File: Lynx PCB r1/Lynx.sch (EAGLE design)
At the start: 105 parts, among them IC3 ICL7660, Q1 8MHz, X1 BU-SMA-V, X2 BU-SMA-V

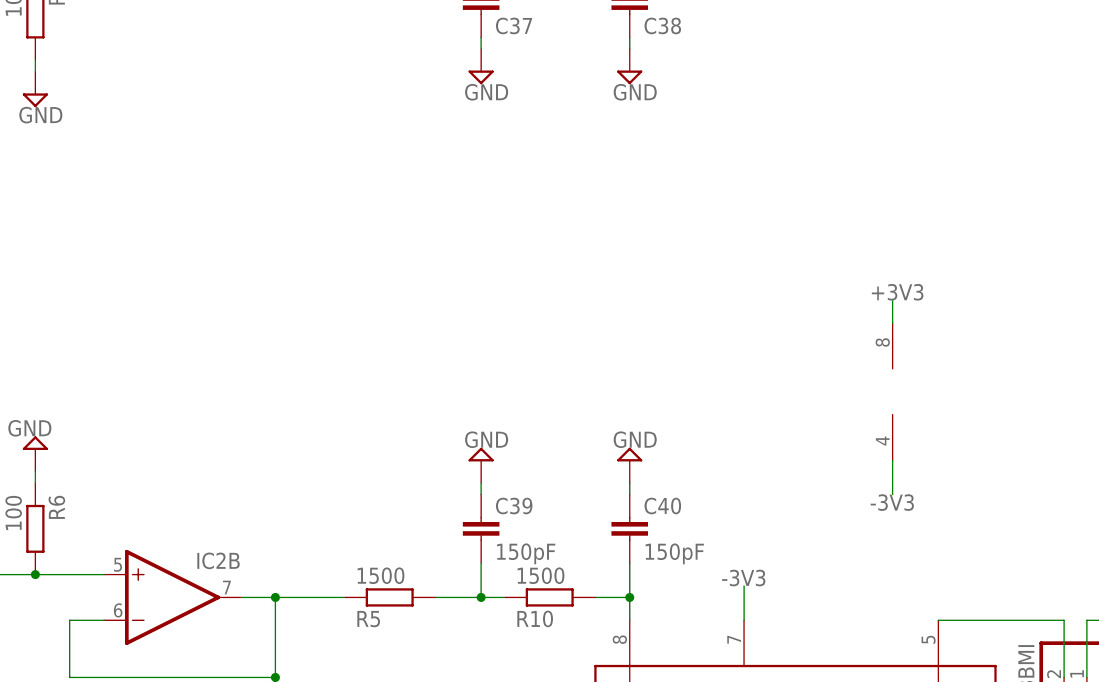
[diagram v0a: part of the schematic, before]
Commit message: All routed
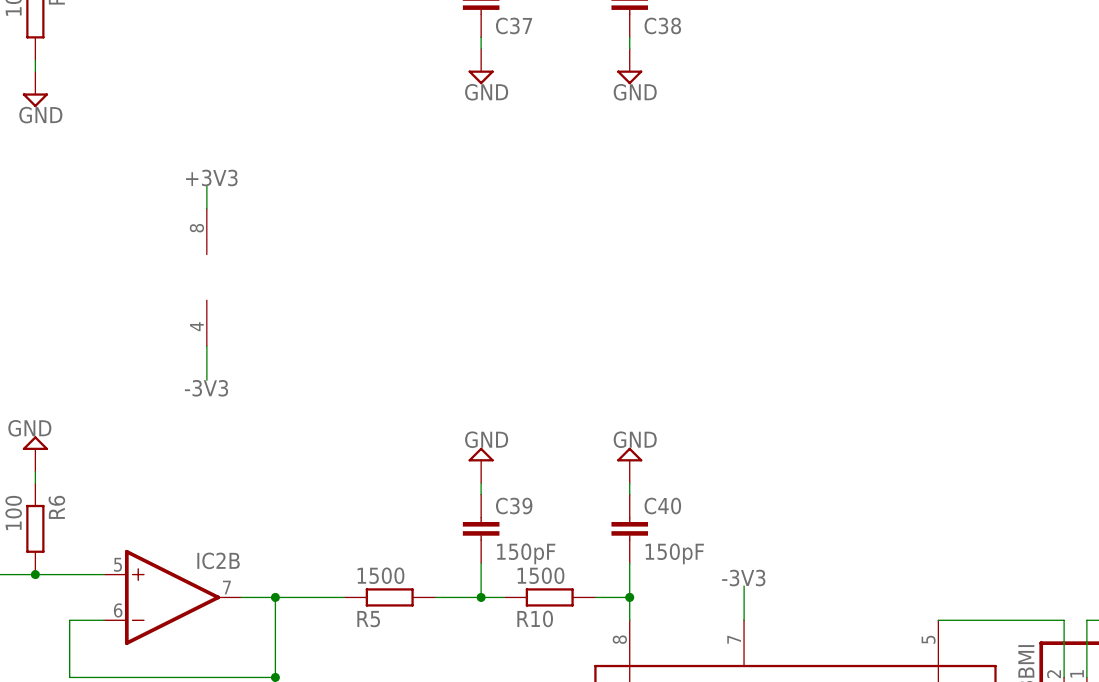
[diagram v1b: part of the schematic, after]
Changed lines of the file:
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@@
 <setting verticaltext="up"/>
 </settings>
-<grid distance="0.05" unitdist="inch" unit="inch" style="lines" multiple="1" display="no" altdistance="0.01" altunitdist="inch" altunit="inch"/>
+<grid distance="0.1" unitdist="inch" unit="inch" style="lines" multiple="1" display="no" altdistance="0.01" altunitdist="inch" altunit="inch"/>
 <layers>
-<layer number="1" name="Top" color="4" fill="1" visible="yes" active="no"/>
-<layer number="2" name="Route2" color="1" fill="3" visible="yes" active="no"/>
-<layer number="3" name="Route3" color="4" fill="3" visible="yes" active="no"/>
-<layer number="4" name="Route4" color="1" fill="4" visible="yes" active="no"/>
-<layer number="5" name="Route5" color="4" fill="4" visible="yes" active="no"/>
-<layer number="6" name="Route6" color="1" fill="8" visible="yes" active="no"/>
-<layer number="7" name="Route7" color="4" fill="8" visible="yes" active="no"/>
-<layer number="8" name="Route8" color="1" fill="2" visible="yes" active="no"/>
-<layer number="9" name="Route9" color="4" fill="2" visible="yes" active="no"/>
-<layer number="10" name="Route10" color="1" fill="7" visible="yes" active="no"/>
-<layer number="11" name="Route11" color="4" fill="7" visible="yes" active="no"/>
-<layer number="12" name="Route12" color="1" fill="5" visible="yes" active="no"/>
-<layer number="13" name="Route13" color="4" fill="5" visible="yes" active="no"/>
-<layer number="14" name="Route14" color="1" fill="6" visible="yes" active="no"/>
-<layer number="15" name="Route15" color="4" fill="6" visible="yes" active="no"/>
-<layer number="16" name="Bottom" color="1" fill="1" visible="yes" active="no"/>
-<layer number="17" name="Pads" color="2" fill="1" visible="yes" active="no"/>
-<layer number="18" name="Vias" color="2" fill="1" visible="yes" active="no"/>
-<layer number="19" name="Unrouted" color="6" fill="1" visible="yes" active="no"/>
-<layer number="20" name="Dimension" color="15" fill="1" visible="yes" active="no"/>
-<layer number="21" name="tPlace" color="7" fill="1" visible="yes" active="no"/>
-<layer number="22" name="bPlace" color="7" fill="1" visible="yes" active="no"/>
-<layer number="23" name="tOrigins" color="15" fill="1" visible="yes" active="no"/>
-<layer number="24" name="bOrigins" color="15" fill="1" visible="yes" active="no"/>
-<layer number="25" name="tNames" color="7" fill="1" visible="yes" active="no"/>
-<layer number="26" name="bNames" color="7" fill="1" visible="yes" active="no"/>
-<layer number="27" name="tValues" color="7" fill="1" visible="yes" active="no"/>
-<layer number="28" name="bValues" color="7" fill="1" visible="yes" active="no"/>
+<layer number="1" name="Top" color="4" fill="1" visible="no" active="no"/>
+<layer number="2" name="Route2" color="1" fill="3" visible="no" active="no"/>
+<layer number="3" name="Route3" color="4" fill="3" visible="no" active="no"/>
+<layer number="4" name="Route4" color="1" fill="4" visible="no" active="no"/>
+<layer number="5" name="Route5" color="4" fill="4" visible="no" active="no"/>
+<layer number="6" name="Route6" color="1" fill="8" visible="no" active="no"/>
+<layer number="7" name="Route7" color="4" fill="8" visible="no" active="no"/>
+<layer number="8" name="Route8" color="1" fill="2" visible="no" active="no"/>
+<layer number="9" name="Route9" color="4" fill="2" visible="no" active="no"/>
+<layer number="10" name="Route10" color="1" fill="7" visible="no" active="no"/>
+<layer number="11" name="Route11" color="4" fill="7" visible="no" active="no"/>
+<layer number="12" name="Route12" color="1" fill="5" visible="no" active="no"/>
+<layer number="13" name="Route13" color="4" fill="5" visible="no" active="no"/>
+<layer number="14" name="Route14" color="1" fill="6" visible="no" active="no"/>
+<layer number="15" name="Route15" color="4" fill="6" visible="no" active="no"/>
+<layer number="16" name="Bottom" color="1" fill="1" visible="no" active="no"/>
+<layer number="17" name="Pads" color="2" fill="1" visible="no" active="no"/>
+<layer number="18" name="Vias" color="2" fill="1" visible="no" active="no"/>
+<layer number="19" name="Unrouted" color="6" fill="1" visible="no" active="no"/>
+<layer number="20" name="Dimension" color="15" fill="1" visible="no" active="no"/>
+<layer number="21" name="tPlace" color="7" fill="1" visible="no" active="no"/>
+<layer number="22" name="bPlace" color="7" fill="1" visible="no" active="no"/>
+<layer number="23" name="tOrigins" color="15" fill="1" visible="no" active="no"/>
+<layer number="24" name="bOrigins" color="15" fill="1" visible="no" active="no"/>
+<layer number="25" name="tNames" color="7" fill="1" visible="no" active="no"/>
+<layer number="26" name="bNames" color="7" fill="1" visible="no" active="no"/>
+<layer number="27" name="tValues" color="7" fill="1" visible="no" active="no"/>
+<layer number="28" name="bValues" color="7" fill="1" visible="no" active="no"/>
 <layer number="29" name="tStop" color="7" fill="3" visible="no" active="no"/>
 <layer number="30" name="bStop" color="7" fill="6" visible="no" active="no"/>
@@
 <layer number="35" name="tGlue" color="7" fill="4" visible="no" active="no"/>
 <layer number="36" name="bGlue" color="7" fill="5" visible="no" active="no"/>
-<layer number="37" name="tTest" color="7" fill="1" visible="yes" active="no"/>
-<layer number="38" name="bTest" color="7" fill="1" visible="yes" active="no"/>
+<layer number="37" name="tTest" color="7" fill="1" visible="no" active="no"/>
+<layer number="38" name="bTest" color="7" fill="1" visible="no" active="no"/>
 <layer number="39" name="tKeepout" color="4" fill="11" visible="no" active="no"/>
 <layer number="40" name="bKeepout" color="1" fill="11" visible="no" active="no"/>
@@
 <layer number="44" name="Drills" color="7" fill="1" visible="no" active="no"/>
 <layer number="45" name="Holes" color="7" fill="1" visible="no" active="no"/>
-<layer number="46" name="Milling" color="3" fill="1" visible="yes" active="no"/>
-<layer number="47" name="Measures" color="7" fill="1" visible="yes" active="no"/>
-<layer number="48" name="Document" color="7" fill="1" visible="yes" active="no"/>
-<layer number="49" name="Reference" color="7" fill="1" visible="yes" active="no"/>
-<layer number="50" name="dxf" color="7" fill="1" visible="yes" active="no"/>
-<layer number="51" name="tDocu" color="7" fill="1" visible="yes" active="no"/>
-<layer number="52" name="bDocu" color="7" fill="1" visible="yes" active="no"/>
-<layer number="53" name="tGND_GNDA" color="7" fill="9" visible="yes" active="no"/>
-<layer number="54" name="bGND_GNDA" color="1" fill="9" visible="yes" active="no"/>
-<layer number="56" name="wert" color="7" fill="1" visible="yes" active="no"/>
+<layer number="46" name="Milling" color="3" fill="1" visible="no" active="no"/>
+<layer number="47" name="Measures" color="7" fill="1" visible="no" active="no"/>
+<layer number="48" name="Document" color="7" fill="1" visible="no" active="no"/>
+<layer number="49" name="Reference" color="7" fill="1" visible="no" active="no"/>
+<layer number="50" name="dxf" color="7" fill="1" visible="no" active="no"/>
+<layer number="51" name="tDocu" color="7" fill="1" visible="no" active="no"/>
+<layer number="52" name="bDocu" color="7" fill="1" visible="no" active="no"/>
+<layer number="53" name="tGND_GNDA" color="7" fill="9" visible="no" active="no"/>
+<layer number="54" name="bGND_GNDA" color="1" fill="9" visible="no" active="no"/>
+<layer number="56" name="wert" color="7" fill="1" visible="no" active="no"/>
 <layer number="91" name="Nets" color="2" fill="1" visible="yes" active="yes"/>
 <layer number="92" name="Busses" color="1" fill="1" visible="yes" active="yes"/>
@@
 <instance part="IC2" gate="A" x="-2.54" y="7.62" rot="MR180"/>
 <instance part="IC2" gate="B" x="-2.54" y="-66.04"/>
-<instance part="IC2" gate="P" x="77.47" y="-43.18"/>
+<instance part="IC2" gate="P" x="1.27" y="-30.48"/>
 <instance part="R4" gate="G$1" x="24.13" y="7.62"/>
 <instance part="R9" gate="G$1" x="39.37" y="7.62"/>
@@
 <segment>
 <pinref part="IC2" gate="P" pin="V+"/>
-<wire x1="77.47" y1="-35.56" x2="77.47" y2="-33.02" width="0.1524" layer="91"/>
-<label x="74.93" y="-33.02" size="1.778" layer="95"/>
+<wire x1="1.27" y1="-22.86" x2="1.27" y2="-20.32" width="0.1524" layer="91"/>
+<label x="-1.27" y="-20.32" size="1.778" layer="95"/>
 </segment>
 <segment>
@@
 <segment>
 <pinref part="IC2" gate="P" pin="V-"/>
-<wire x1="77.47" y1="-50.8" x2="77.47" y2="-54.61" width="0.1524" layer="91"/>
-<label x="80.01" y="-54.61" size="1.778" layer="95" rot="R180"/>
-</segment>
-<segment>
+<wire x1="1.27" y1="-38.1" x2="1.27" y2="-41.91" width="0.1524" layer="91"/>
+<label x="3.81" y="-41.91" size="1.778" layer="95" rot="R180"/>
+</segment>
+<segment>
